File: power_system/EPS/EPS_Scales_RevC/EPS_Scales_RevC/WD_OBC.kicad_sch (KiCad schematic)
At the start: 36 parts, among them J18 Conn_01x04, U14 TLV1704

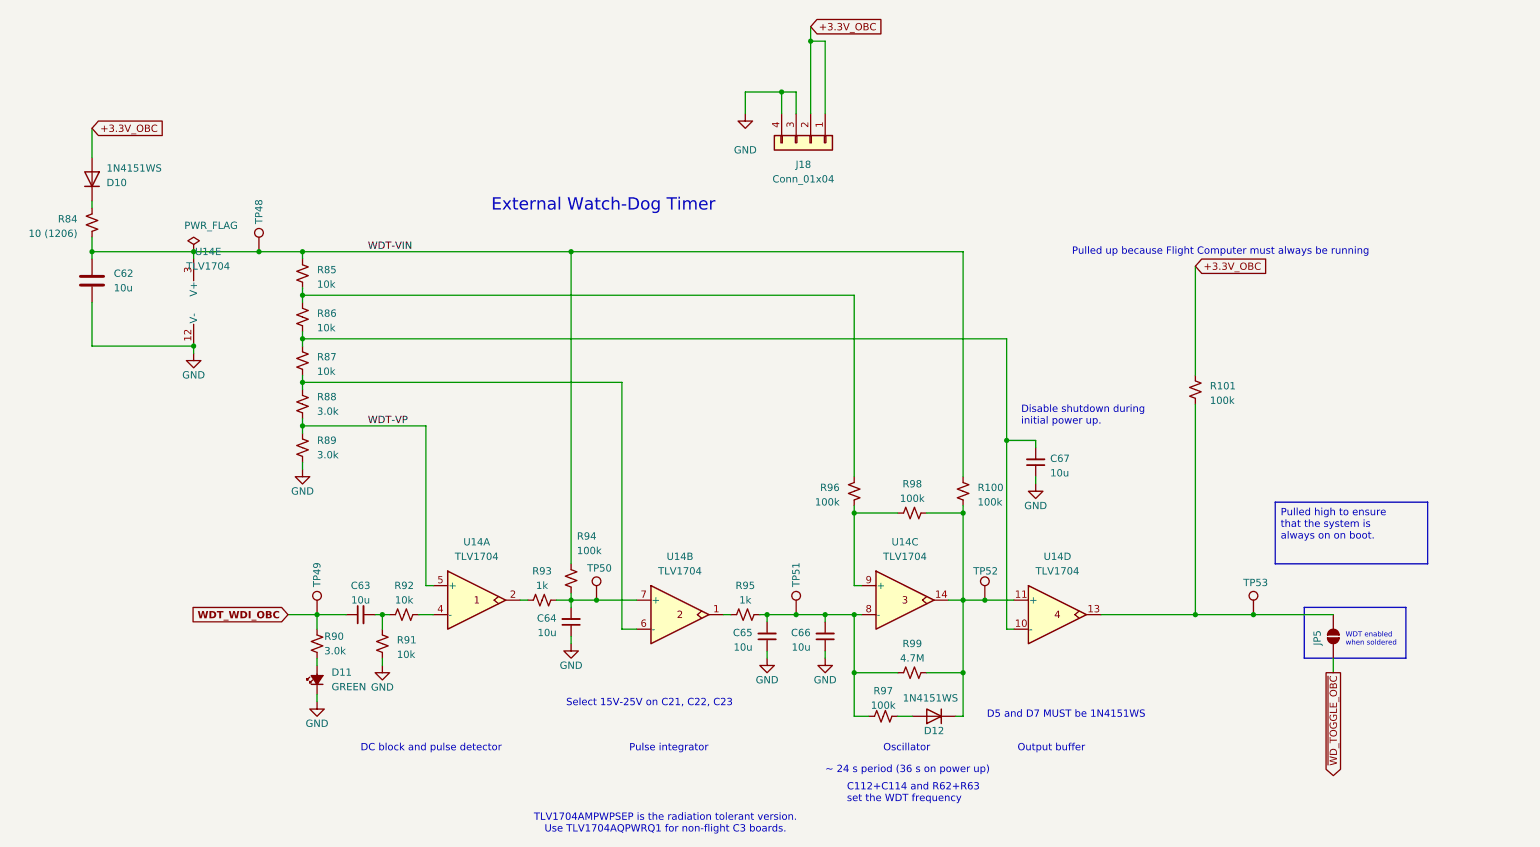
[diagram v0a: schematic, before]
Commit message: Revert "Luca branch v2"
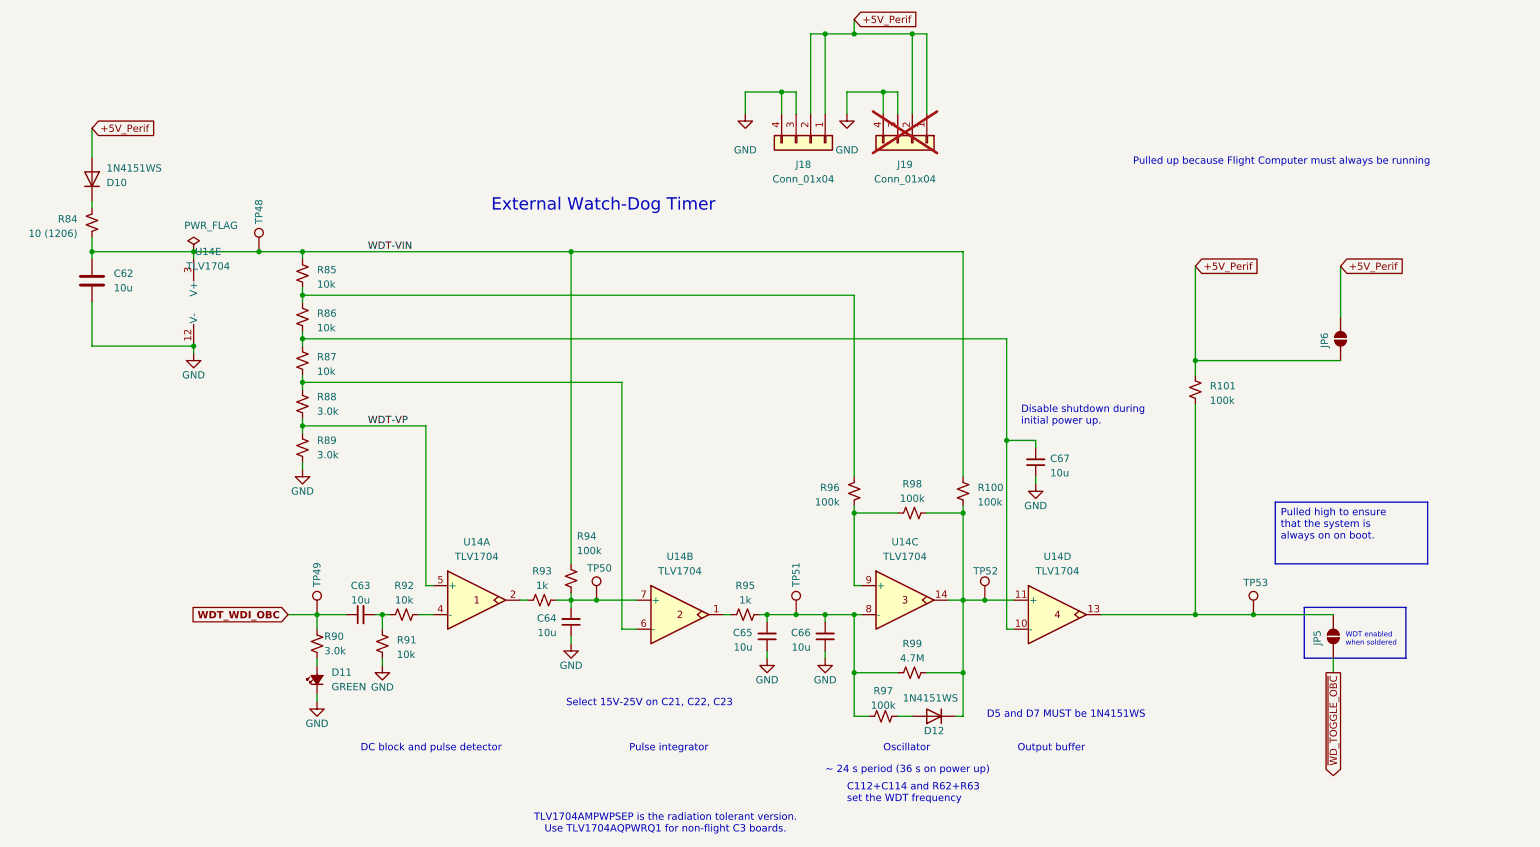
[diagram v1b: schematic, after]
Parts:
- added J19: Conn_01x04, Connector_PinSocket_2.54mm:PinSocket_1x04_P2.54mm_Vertical, symbol Connector_Generic:Conn_01x04
- added JP6: SolderJumper_2_Open, Jumper:SolderJumper-2_P1.3mm_Open_RoundedPad1.0x1.5mm, symbol Jumper:SolderJumper_2_Open
- D10, D12: footprint RevC Footprints:SODFL2512X100N -> Diode_SMD:D_SOD-323
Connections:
- net GND: now also J19.3 (Pin_3), J19.4 (Pin_4)
- net +3.3V_OBC renamed +5V_Perif
- net +5V_Perif: now also J19.1 (Pin_1), J19.2 (Pin_2), JP6.1 (A), JP6.2 (B)
